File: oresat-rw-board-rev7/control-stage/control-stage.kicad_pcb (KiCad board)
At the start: 6 copper layers, 40 x 39.5 mm, 68 parts, among them J1 MEZZ, J2 10132797-021100LF, J3 10132797-021100LF, J4 10132797-021100LF, J5 Hirose_FH12-10S-0.5SH, Q1 TPN4R712MD,L1Q, U1 ADP7156ACPZ, U2 TLV62569DRL, U3 STM32G474RBTx, U5 TCAN330, Y1 Crystal_GND24

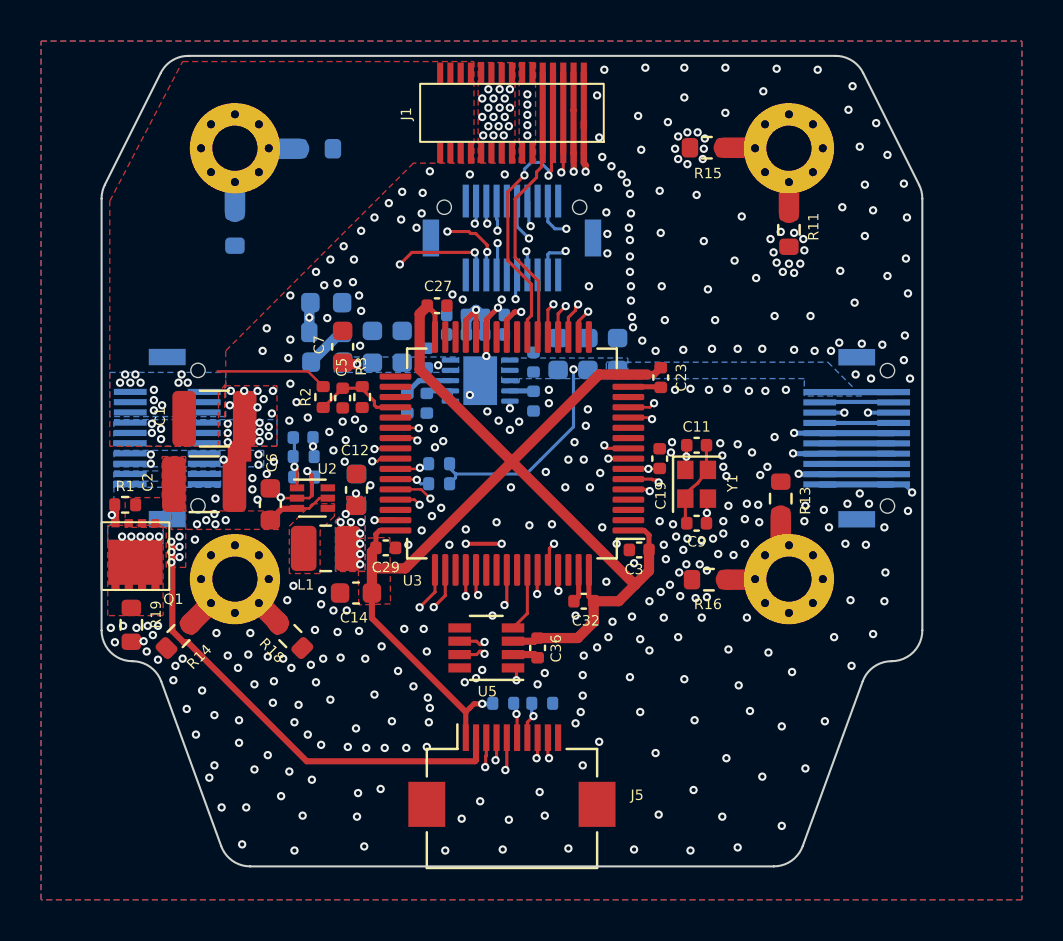
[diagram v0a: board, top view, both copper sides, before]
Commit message: Move rev-7 to oresat-acs-board-rev7
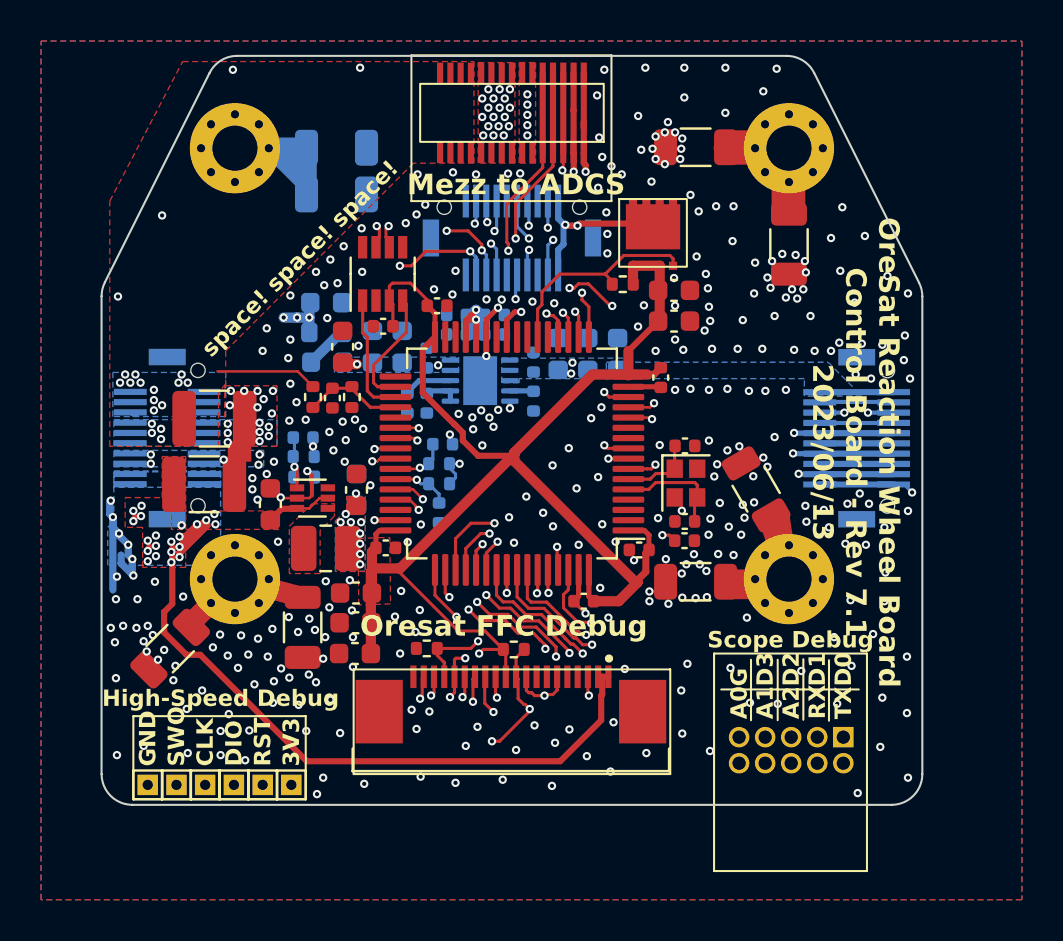
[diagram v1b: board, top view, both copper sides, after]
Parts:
- removed J5: Hirose_FH12-10S-0.5SH, Connector_FFC-FPC:Hirose_FH12-10S-0.5SH_1x10-1MP_P0.50mm_Horizontal
- removed R19: THJP0603ABT1, Resistor_SMD:R_0603_1608Metric
- added C21: 22u, Capacitor_SMD:C_0603_1608Metric, F.Cu at (105.2, 62.0)
- added C30: 22u, Capacitor_SMD:C_0603_1608Metric, F.Cu at (89.7, 76.8)
- added C31: 22u, Capacitor_SMD:C_0603_1608Metric, F.Cu at (89.7, 78.2)
- added C33: 22u, Capacitor_SMD:C_0603_1608Metric, F.Cu at (105.2, 60.5)
- added C34: 1u, Capacitor_SMD:C_0402_1005Metric, B.Cu at (93.8, 71.4)
- added C39: 1u, Capacitor_SMD:C_0402_1005Metric, B.Cu at (93.9, 68.0)
- added J6: J-TE-Debug-2-1734592-0, rev-7-footprints:J-TE_2-1734592-0, F.Cu at (97.2, 81.1)
- added J7: PROBE, Connector_PinHeader_1.27mm:PinHeader_2x05_P1.27mm_Horizontal, F.Cu at (113.5, 82.3)
- added TP1: TestPoint_Alt, TestPoint:TestPoint_THTPad_1.0x1.0mm_Drill0.5mm, F.Cu at (81.0, 84.7)
- added TP2: TestPoint_Alt, TestPoint:TestPoint_THTPad_1.0x1.0mm_Drill0.5mm, F.Cu at (79.5, 84.7)
- added TP3: TestPoint_Alt, TestPoint:TestPoint_THTPad_1.0x1.0mm_Drill0.5mm, F.Cu at (83.8, 84.7)
- added TP4: TestPoint_Alt, TestPoint:TestPoint_THTPad_1.0x1.0mm_Drill0.5mm, F.Cu at (82.3, 84.7)
- added TP5: TestPoint_Alt, TestPoint:TestPoint_THTPad_1.0x1.0mm_Drill0.5mm, F.Cu at (85.2, 84.7)
- added TP6: TestPoint_Alt, TestPoint:TestPoint_THTPad_1.0x1.0mm_Drill0.5mm, F.Cu at (86.5, 84.7)
- C11, C9: value 20p -> 18p
- H1: footprint rev-7-footprints:top-board-def -> rev-7-footprints:top-board-def-rev7.1
- R1: value 100k -> 100k/1%
- R11, R12, R13, R14, R15, R16, R17, R18: value THJP0603ABT1 -> THJP1206ABT1; footprint Resistor_SMD:R_0603_1608Metric -> Resistor_SMD:R_1206_3216Metric
- R6, R7: moved to F.Cu
- U3: value STM32G474RBTx -> STM32G474RET3
- moved Q1 29.7 mm to (104.2, 57.8), turned to 0 degrees
- moved R1 26.5 mm to (102.7, 60.2), turned to 0 degrees
- moved U5 18.9 mm to (91.0, 59.8), turned to 90 degrees
- moved C36 17.4 mm to (91.0, 62.3), turned to 180 degrees
- moved R7 6.23 mm to (93.2, 78.0), turned to 180 degrees
- moved R17 5.23 mm to (88.8, 55.9), turned to 0 degrees
- moved C19 4.18 mm to (105.7, 72.8), turned to 0 degrees
- moved R6 2.68 mm to (97.4, 78.0)
- moved R13 1.28 mm to (109.2, 70.2), turned to 120 degrees
- moved R12 1.00 mm to (88.8, 53.6)
- moved R18 0.74 mm to (87.1, 77.0), turned to -90 degrees
- moved R14 0.73 mm to (80.6, 78.0)
- moved R11 0.70 mm to (110.8, 58.3)
- moved R16 0.66 mm to (106.2, 74.8)
- moved C9 0.59 mm to (105.7, 71.8)
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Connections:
- net Net-(C10-Pad1) renamed /5V_FILT
- J2 pad 10: +5V_SW -> +5V
- J2 pad 11: +5V_SW -> +5V
- J2 pad 12: +5V_SW -> +5V
- J2 pad 9: +5V_SW -> +5V
- J3 pad 10: GND -> /+3V3_SW
- J3 pad 11: GND -> /+3V3_SW
- Q1 pad 1: +5V -> +3V3
- Q1 pad 2: /SW_5V -> /SW_3V3
- Q1 pad 3: +5V_SW -> /+3V3_SW
- R1 pad 1: +5V -> /SW_3V3
- R1 pad 2: /SW_5V -> +3V3
- U3 pad 14: unconnected-(U3-Pad14) -> /UART_TX
- U3 pad 17: unconnected-(U3-Pad17) -> /UART_RX
- U3 pad 18: /SPI_nCS -> /SCOPE0
- U3 pad 19: /SPI_SCK -> /SCOPE1
- U3 pad 20: /SPI_MISO -> /SCOPE2
- U3 pad 21: /SPI_MOSI -> unconnected-(U3-PA7-Pad21)
- U3 pad 22: /UART_TX -> /SW_3V3
- U3 pad 23: /UART_RX -> unconnected-(U3-PC5-Pad23)
- U3 pad 34: unconnected-(U3-Pad34) -> /CAN_RX
- U3 pad 35: unconnected-(U3-Pad35) -> /CAN_TX
- U3 pad 51: unconnected-(U3-Pad51) -> /SPI_nCS
- U3 pad 52: /DEBUG_TX -> /SPI_SCK
- U3 pad 53: /DEBUG_RX -> /SPI_MISO
- U3 pad 54: unconnected-(U3-Pad54) -> /SPI_MOSI
- U3 pad 55: unconnected-(U3-Pad55) -> /DEBUG3
- U3 pad 57: unconnected-(U3-Pad57) -> /DEBUG2
- U3 pad 58: /CAN_RX -> /DEBUG1
- U3 pad 59: /CAN_TX -> /DEBUG_TX
- U3 pad 60: /SW_5V -> /DEBUG_RX
- U3 pad 62: unconnected-(U3-Pad62) -> /DEBUG0
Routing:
- net /SCOPE2: track 0.00 -> 39.6 mm, vias 0 -> 3
- net /SCOPE1: track 0.00 -> 37.3 mm, vias 0 -> 3
- net /SCOPE0: track 0.00 -> 34.9 mm, vias 0 -> 3
- net /UART_TX: track 13.9 -> 46.6 mm, vias 0 -> 5
- net +3V3: track 70.0 -> 100.5 mm
- net /SW_5V: track 29.8 -> 0.00 mm, vias 4 -> 0
- net /UART_RX: track 15.9 -> 43.6 mm, vias 2 -> 3
- net +5V: track 31.7 -> 55.3 mm, vias 17 -> 28
- net /CAN_P: track 37.8 -> 17.3 mm
- net /CAN_N: track 37.3 -> 17.7 mm
- net /CHASSIS: track 25.1 -> 44.1 mm
- net /DEBUG1: track 0.00 -> 18.8 mm, vias 0 -> 1
- net /DEBUG3: track 0.00 -> 18.7 mm, vias 0 -> 1
- net /DEBUG2: track 0.00 -> 18.5 mm, vias 0 -> 1
- net /DEBUG0: track 0.00 -> 18.2 mm, vias 0 -> 1
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- added copper zone on B.Cu, net +5V
- removed copper zone on B.Cu, net +5V_SW
- removed copper zone on F.Cu, net +5V_SW
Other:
- board size 40 x 39.5 mm -> 40 x 36.5 mm
- board text added: "3V3"
- board text added: "A0"
- board text added: "A1"
- board text added: "A2"
- board text added: "CLK"
- board text added: "D0"
- board text added: "D1"
- board text added: "D2"
- board text added: "D3"
- board text added: "DIO"
- board text added: "Digital"
- board text added: "Do we need more capacitors?"
- board text added: "F.Cu -> Power In1.Cu -> Digital GND In2.Cu -> Digital Signals In3.Cu -> Analog Signals In4.Cu -> Analog GND B.Cu -> Analog Power"
- board text added: "G"
- board text added: "GND"
- board text added: "High-Speed Debug"
- board text added: "Maybe the aliens will have STM32s in stock..."
- board text added: "Mezz to ADCS"
- board text added: "OreSat Reaction Wheel Board Control Board - Rev 7.1 2023/06/13"
- board text added: "Oresat FFC Debug"
- board text added: "RST"
- board text added: "RX"
- board text added: "SWO"
- board text added: "Scope Debug"
- board text added: "TX"
- board text added: "Wait, this thing's going"
- board text added: "space! space! space!"
- board text added: "where?"
- board text removed: "F.Cu -> Power In1.Cu -> Digital Ground In2.Cu -> Digital Signals In3.Cu -> Analog Signals In4.Cu -> Analog GND B.Cu -> Analog Power"
